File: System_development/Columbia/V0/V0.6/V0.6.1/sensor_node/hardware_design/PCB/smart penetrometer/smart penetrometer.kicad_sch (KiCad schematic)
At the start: 29 parts, among them J2 Conn_01x02, J3 Conn_01x02, J4 Conn_01x07_Female, J5 Conn_02x04, U1 LM321, U2 ADP124ARHZ-3.3-R7, U4 DS3231M, U5 BME260, U7 ADS1115IDGS

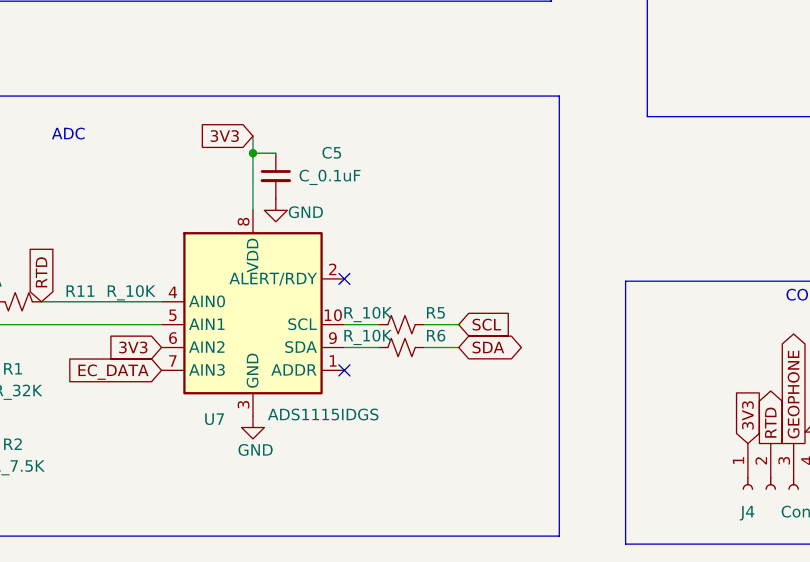
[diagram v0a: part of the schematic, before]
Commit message: V0.6.1 update
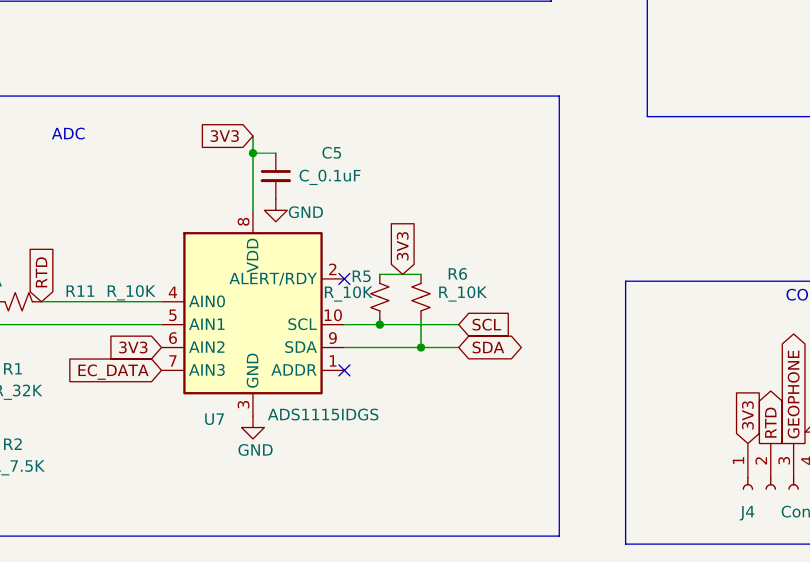
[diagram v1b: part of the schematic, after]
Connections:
- net 3V3: now also R5.1, R6.1
- net SCL: now also R5.2, U7.10 (SCL); no longer R5.1
- net SDA: now also R6.2, U7.9 (SDA); no longer R6.1
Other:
- moved on the sheet: R5, R6
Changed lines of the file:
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@@
 	)
 	(junction
+		(at 103.632 172.466)
+		(diameter 0)
+		(color 0 0 0 0)
+	)
+	(junction
 		(at 46.99 113.665)
 		(diameter 0)
@@
 	)
 	(junction
+		(at 99.06 169.926)
+		(diameter 0)
+		(color 0 0 0 0)
+	)
+	(junction
 		(at 50.165 116.205)
 		(diameter 0)
@@
 	(wire
 		(pts
+			(xy 99.06 169.418) (xy 99.06 169.926)
+		)
+		(stroke
+			(width 0)
+			(type default)
+		)
+	)
+	(wire
+		(pts
 			(xy 151.13 44.196) (xy 153.67 44.196)
 		)
@@
 	(wire
 		(pts
-			(xy 95.123 172.466) (xy 98.933 172.466)
+			(xy 103.632 169.418) (xy 103.632 172.466)
+		)
+		(stroke
+			(width 0)
+			(type default)
+		)
+	)
+	(wire
+		(pts
+			(xy 95.123 172.466) (xy 103.632 172.466)
 		)
 		(stroke
@@
 		)
 	)
+	(wire
+		(pts
+			(xy 99.06 169.926) (xy 107.823 169.926)
+		)
+		(stroke
+			(width 0)
+			(type default)
+		)
+	)
 	(polyline
 		(pts
@@
 		)
 	)
-	(polyline
+	(wire
 		(pts
-			(xy 126.365 194.31) (xy 126.365 165.1)
+			(xy 103.632 172.466) (xy 107.823 172.466)
 		)
 		(stroke
@@
 		)
 	)
-	(wire
+	(polyline
 		(pts
-			(xy 84.963 150.876) (xy 87.503 150.876)
+			(xy 126.365 194.31) (xy 126.365 165.1)
 		)
 		(stroke
@@
 	(wire
 		(pts
-			(xy 104.013 169.926) (xy 107.823 169.926)
+			(xy 84.963 150.876) (xy 87.503 150.876)
 		)
 		(stroke
@@
 	(wire
 		(pts
-			(xy 95.123 169.926) (xy 98.933 169.926)
-		)
-		(stroke
-			(width 0)
-			(type default)
-		)
-	)
-	(wire
-		(pts
-			(xy 104.013 172.466) (xy 107.823 172.466)
+			(xy 95.123 169.926) (xy 99.06 169.926)
 		)
 		(stroke
@@
 		)
 	)
+	(wire
+		(pts
+			(xy 99.06 164.338) (xy 103.632 164.338)
+		)
+		(stroke
+			(width 0)
+			(type default)
+		)
+	)
 	(rectangle
 		(start 42.545 27.305)
@@
 		)
 	)
+	(global_label "3V3"
+		(shape input)
+		(at 101.6 164.338 90)
+		(fields_autoplaced yes)
+		(effects
+			(font
+				(size 1.27 1.27)
+			)
+			(justify left)
+		)
+		(property "Intersheetrefs" "${INTERSHEET_REFS}"
+			(at 101.6 157.8452 90)
+			(effects
+				(font
+					(size 1.27 1.27)
+				)
+				(justify left)
+				(hide yes)
+			)
+		)
+	)
 	(global_label "CLK"
 		(shape output)
@@
 	(symbol
 		(lib_id "Device:R_Small_US")
-		(at 101.473 169.926 270)
+		(at 99.06 166.878 0)
 		(unit 1)
 		(exclude_from_sim no)
@@
 		(dnp no)
 		(property "Reference" "R5"
-			(at 105.283 168.656 90)
+			(at 97.028 164.592 0)
 			(effects
 				(font
@@
 		)
 		(property "Value" "R_10K"
-			(at 97.663 168.656 90)
+			(at 95.504 166.37 0)
 			(effects
 				(font
@@
 		)
 		(property "Footprint" "Resistor_SMD:R_1206_3216Metric"
-			(at 101.473 169.926 0)
+			(at 99.06 166.878 0)
 			(effects
 				(font
@@
 		)
 		(property "Datasheet" "~"
-			(at 101.473 169.926 0)
+			(at 99.06 166.878 0)
 			(effects
 				(font
@@
 		)
 		(property "Description" ""
-			(at 101.473 169.926 0)
+			(at 99.06 166.878 0)
 			(effects
 				(font
@@
 	(symbol
 		(lib_id "Device:R_Small_US")
-		(at 101.473 172.466 270)
+		(at 103.632 166.878 0)
+		(mirror y)
 		(unit 1)
 		(exclude_from_sim no)
@@
 		(dnp no)
 		(property "Reference" "R6"
-			(at 105.283 171.196 90)
+			(at 107.696 164.338 0)
 			(effects
 				(font
@@
 		)
 		(property "Value" "R_10K"
-			(at 97.663 171.196 90)
+			(at 108.204 166.37 0)
 			(effects
 				(font
@@
 		)
 		(property "Footprint" "Resistor_SMD:R_1206_3216Metric"
-			(at 101.473 172.466 0)
+			(at 103.632 166.878 0)
 			(effects
 				(font
@@
 		)
 		(property "Datasheet" "~"
-			(at 101.473 172.466 0)
+			(at 103.632 166.878 0)
 			(effects
 				(font
@@
 		)
 		(property "Description" ""
-			(at 101.473 172.466 0)
+			(at 103.632 166.878 0)
 			(effects
 				(font
